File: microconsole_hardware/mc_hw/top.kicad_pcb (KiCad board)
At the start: 2 copper layers, 161 x 96 mm, 110 parts, among them J1 USB_C_Receptacle_USB2.0_16P, Q1 Q_PMOS_GSD, SW1 SW_Nidec_CAS-120A1, SW10 TL3301NF160QG, SW11 TL3301NF160QG, SW12 TL3301NF160QG, SW13 TL3301NF160QG, SW14 TL3301NF160QG, SW15 TL3301NF160QG, SW16 Joystick, SW17 Joystick, SW2 TL3301NF160QG, SW3 TL3301NF160QG, SW4 TL3301NF160QG, SW5 TL3301NF160QG, SW6 TL3301NF160QG, SW7 TL3301NF160QG, SW8 TL3301NF160QG, SW9 TL3301NF160QG, U1 MCP73833_MSOP, U2 S2B-PH-K-S, U3 MCP23017-E/SO, U4 ADS7828E/2K5, U5 PCM5102APWR, U6 PAM8302AADCR, U7 PAM8406DR

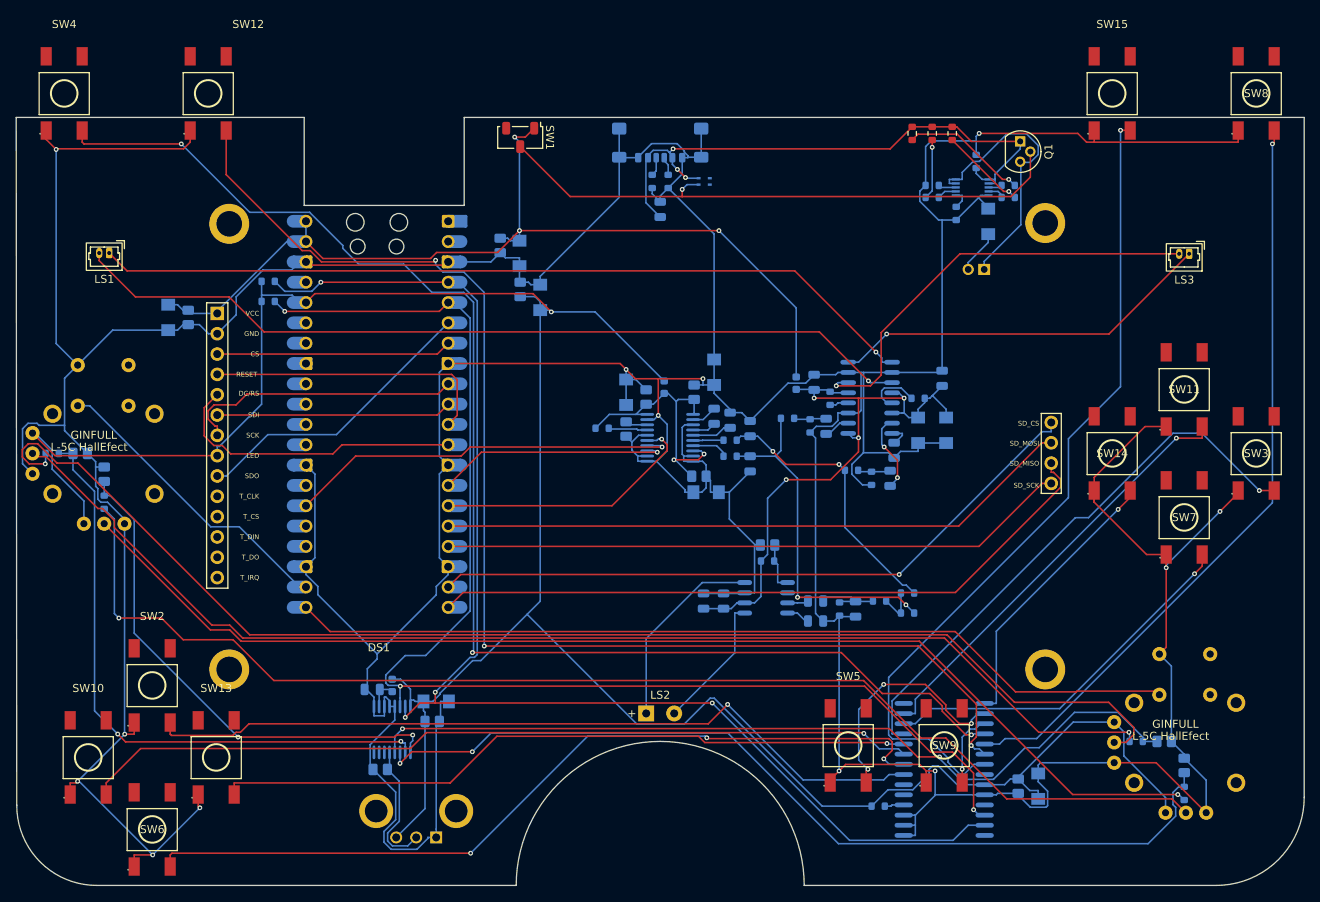
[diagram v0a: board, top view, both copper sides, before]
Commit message: clean up tracks
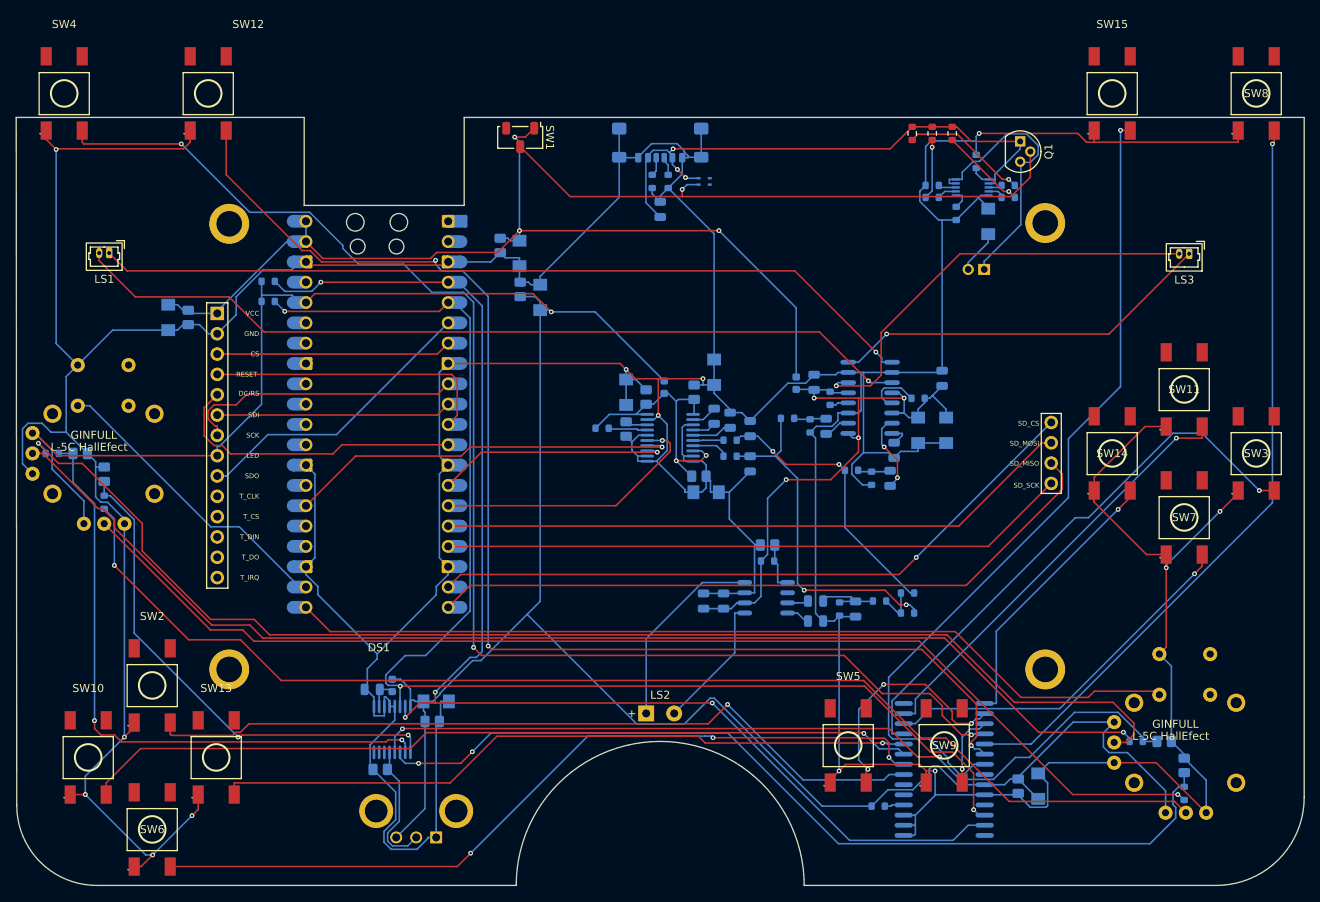
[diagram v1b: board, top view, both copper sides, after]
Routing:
- net IO1 / Left Stick Y: track 163.1 -> 159.4 mm
- net IO0 / Left Stick X: track 157.9 -> 154.3 mm
- net GND: track 906.4 -> 903.9 mm
- net MCP GPA1 / DPAD - DOWN: track 103.5 -> 101.0 mm
- net 3v3: track 315.9 -> 317.8 mm
- net FILTERED - IO1 / Left Stick Y: track 76.8 -> 78.2 mm
- net GPIO11 / MAX LRC: track 34.6 -> 35.4 mm
- net DAC_R: track 44.0 -> 43.3 mm
- net GPIO14 / SD SCK: track 85.4 -> 84.7 mm
- net GPIO2 / MCP|ADC SDA: track 162.5 -> 163.1 mm
- net FILTERED - IO0 / Left Stick X: track 63.5 -> 63.0 mm
- net GPIO16 / Left Stick: track 112.1 -> 112.6 mm
